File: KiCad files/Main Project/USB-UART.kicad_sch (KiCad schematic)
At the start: 6 parts, among them U3 CH340C

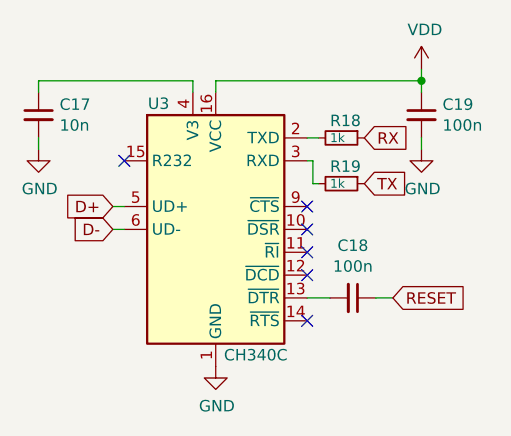
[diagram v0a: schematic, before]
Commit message: shematic update
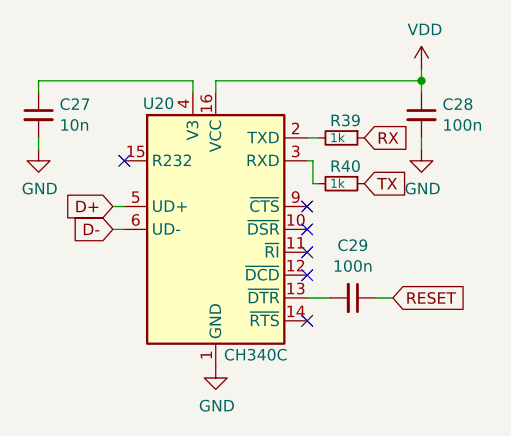
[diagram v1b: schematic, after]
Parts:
- renumbered C17 to C27, C19 to C28, C18 to C29, R18 to R39, R19 to R40, U3 to U20
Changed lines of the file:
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@@
   (symbol (lib_id "Interface_USB:CH340C") (at 140.97 83.82 0) (unit 1)
     (in_bom yes) (on_board yes)
-    (property "Reference" "U3" (id 0) (at 134.62 69.85 0))
+    (property "Reference" "U20" (id 0) (at 134.62 69.85 0))
     (property "Value" "CH340C" (id 1) (at 145.415 97.79 0))
     (property "Footprint" "Package_SO:SOIC-16_3.9x9.9mm_P1.27mm" (id 2) (at 142.24 97.79 0)
@@
   (symbol (lib_id "Device:C_Small") (at 121.285 71.12 0) (unit 1)
     (in_bom yes) (on_board yes)
-    (property "Reference" "C17" (id 0) (at 123.6218 69.9516 0)
+    (property "Reference" "C27" (id 0) (at 123.6218 69.9516 0)
       (effects (font (size 1.27 1.27)) (justify left))
     )
@@
   (symbol (lib_id "power:GND") (at 121.285 74.93 0) (unit 1)
     (in_bom yes) (on_board yes)
-    (property "Reference" "#PWR073" (id 0) (at 121.285 81.28 0)
+    (property "Reference" "#PWR082" (id 0) (at 121.285 81.28 0)
       (effects (font (size 1.27 1.27)) hide)
     )
@@
   (symbol (lib_id "Device:C_Small") (at 163.83 71.12 0) (unit 1)
     (in_bom yes) (on_board yes)
-    (property "Reference" "C19" (id 0) (at 166.1668 69.9516 0)
+    (property "Reference" "C28" (id 0) (at 166.1668 69.9516 0)
       (effects (font (size 1.27 1.27)) (justify left))
     )
@@
   (symbol (lib_id "power:GND") (at 163.83 74.93 0) (unit 1)
     (in_bom yes) (on_board yes)
-    (property "Reference" "#PWR076" (id 0) (at 163.83 81.28 0)
+    (property "Reference" "#PWR083" (id 0) (at 163.83 81.28 0)
       (effects (font (size 1.27 1.27)) hide)
     )
@@
   (symbol (lib_id "power:GND") (at 140.97 99.06 0) (unit 1)
     (in_bom yes) (on_board yes)
-    (property "Reference" "#PWR074" (id 0) (at 140.97 105.41 0)
+    (property "Reference" "#PWR084" (id 0) (at 140.97 105.41 0)
       (effects (font (size 1.27 1.27)) hide)
     )
@@
   (symbol (lib_id "Device:C_Small") (at 156.21 91.44 270) (unit 1)
     (in_bom yes) (on_board yes)
-    (property "Reference" "C18" (id 0) (at 156.21 85.6234 90))
+    (property "Reference" "C29" (id 0) (at 156.21 85.6234 90))
     (property "Value" "100n" (id 1) (at 156.21 87.9348 90))
     (property "Footprint" "Capacitor_SMD:C_0805_2012Metric" (id 2) (at 156.21 91.44 0)
@@
   (symbol (lib_id "Device:R_Small") (at 154.94 73.66 270) (unit 1)
     (in_bom yes) (on_board yes)
-    (property "Reference" "R18" (id 0) (at 153.67 71.755 90)
+    (property "Reference" "R39" (id 0) (at 153.67 71.755 90)
       (effects (font (size 1.27 1.27)) (justify left))
     )
@@
   (symbol (lib_id "Device:R_Small") (at 154.94 78.74 270) (unit 1)
     (in_bom yes) (on_board yes)
-    (property "Reference" "R19" (id 0) (at 153.67 76.835 90)
+    (property "Reference" "R40" (id 0) (at 153.67 76.835 90)
       (effects (font (size 1.27 1.27)) (justify left))
     )
@@
   (symbol (lib_id "power:VDD") (at 163.83 66.04 0) (unit 1)
     (in_bom yes) (on_board yes)
-    (property "Reference" "#PWR075" (id 0) (at 163.83 69.85 0)
+    (property "Reference" "#PWR081" (id 0) (at 163.83 69.85 0)
       (effects (font (size 1.27 1.27)) hide)
     )

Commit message: update
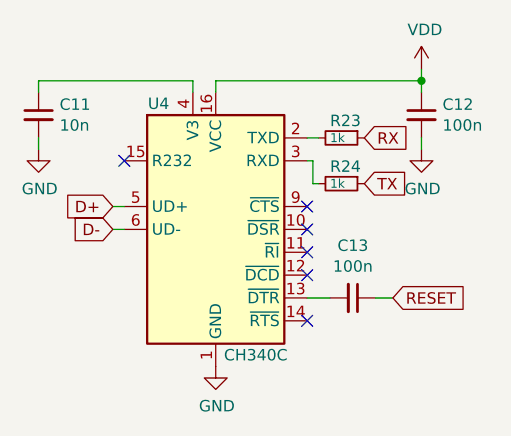
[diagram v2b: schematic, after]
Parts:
- renumbered C27 to C11, C28 to C12, C29 to C13, R39 to R23, R40 to R24, U20 to U4
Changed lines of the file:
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@@
   (symbol (lib_id "Interface_USB:CH340C") (at 140.97 83.82 0) (unit 1)
     (in_bom yes) (on_board yes)
-    (property "Reference" "U20" (id 0) (at 134.62 69.85 0))
+    (property "Reference" "U4" (id 0) (at 134.62 69.85 0))
     (property "Value" "CH340C" (id 1) (at 145.415 97.79 0))
     (property "Footprint" "Package_SO:SOIC-16_3.9x9.9mm_P1.27mm" (id 2) (at 142.24 97.79 0)
@@
   (symbol (lib_id "Device:C_Small") (at 121.285 71.12 0) (unit 1)
     (in_bom yes) (on_board yes)
-    (property "Reference" "C27" (id 0) (at 123.6218 69.9516 0)
+    (property "Reference" "C11" (id 0) (at 123.6218 69.9516 0)
       (effects (font (size 1.27 1.27)) (justify left))
     )
@@
   (symbol (lib_id "power:GND") (at 121.285 74.93 0) (unit 1)
     (in_bom yes) (on_board yes)
-    (property "Reference" "#PWR082" (id 0) (at 121.285 81.28 0)
+    (property "Reference" "#PWR066" (id 0) (at 121.285 81.28 0)
       (effects (font (size 1.27 1.27)) hide)
     )
@@
   (symbol (lib_id "Device:C_Small") (at 163.83 71.12 0) (unit 1)
     (in_bom yes) (on_board yes)
-    (property "Reference" "C28" (id 0) (at 166.1668 69.9516 0)
+    (property "Reference" "C12" (id 0) (at 166.1668 69.9516 0)
       (effects (font (size 1.27 1.27)) (justify left))
     )
@@
   (symbol (lib_id "power:GND") (at 163.83 74.93 0) (unit 1)
     (in_bom yes) (on_board yes)
-    (property "Reference" "#PWR083" (id 0) (at 163.83 81.28 0)
+    (property "Reference" "#PWR067" (id 0) (at 163.83 81.28 0)
       (effects (font (size 1.27 1.27)) hide)
     )
@@
   (symbol (lib_id "power:GND") (at 140.97 99.06 0) (unit 1)
     (in_bom yes) (on_board yes)
-    (property "Reference" "#PWR084" (id 0) (at 140.97 105.41 0)
+    (property "Reference" "#PWR068" (id 0) (at 140.97 105.41 0)
       (effects (font (size 1.27 1.27)) hide)
     )
@@
   (symbol (lib_id "Device:C_Small") (at 156.21 91.44 270) (unit 1)
     (in_bom yes) (on_board yes)
-    (property "Reference" "C29" (id 0) (at 156.21 85.6234 90))
+    (property "Reference" "C13" (id 0) (at 156.21 85.6234 90))
     (property "Value" "100n" (id 1) (at 156.21 87.9348 90))
     (property "Footprint" "Capacitor_SMD:C_0805_2012Metric" (id 2) (at 156.21 91.44 0)
@@
   (symbol (lib_id "Device:R_Small") (at 154.94 73.66 270) (unit 1)
     (in_bom yes) (on_board yes)
-    (property "Reference" "R39" (id 0) (at 153.67 71.755 90)
+    (property "Reference" "R23" (id 0) (at 153.67 71.755 90)
       (effects (font (size 1.27 1.27)) (justify left))
     )
@@
   (symbol (lib_id "Device:R_Small") (at 154.94 78.74 270) (unit 1)
     (in_bom yes) (on_board yes)
-    (property "Reference" "R40" (id 0) (at 153.67 76.835 90)
+    (property "Reference" "R24" (id 0) (at 153.67 76.835 90)
       (effects (font (size 1.27 1.27)) (justify left))
     )
@@
   (symbol (lib_id "power:VDD") (at 163.83 66.04 0) (unit 1)
     (in_bom yes) (on_board yes)
-    (property "Reference" "#PWR081" (id 0) (at 163.83 69.85 0)
+    (property "Reference" "#PWR065" (id 0) (at 163.83 69.85 0)
       (effects (font (size 1.27 1.27)) hide)
     )

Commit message: update
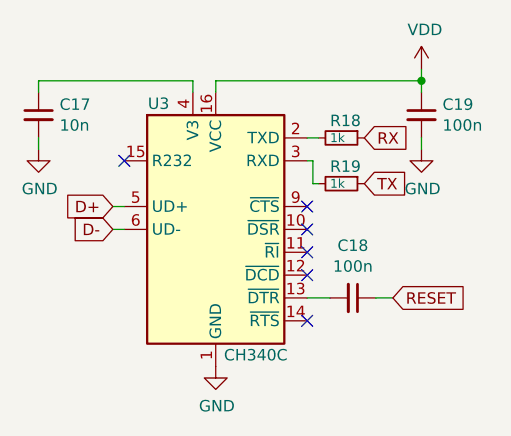
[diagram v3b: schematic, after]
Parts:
- renumbered C11 to C17, C13 to C18, C12 to C19, R23 to R18, R24 to R19, U4 to U3
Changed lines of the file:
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@@
   (symbol (lib_id "Interface_USB:CH340C") (at 140.97 83.82 0) (unit 1)
     (in_bom yes) (on_board yes)
-    (property "Reference" "U4" (id 0) (at 134.62 69.85 0))
+    (property "Reference" "U3" (id 0) (at 134.62 69.85 0))
     (property "Value" "CH340C" (id 1) (at 145.415 97.79 0))
     (property "Footprint" "Package_SO:SOIC-16_3.9x9.9mm_P1.27mm" (id 2) (at 142.24 97.79 0)
@@
   (symbol (lib_id "Device:C_Small") (at 121.285 71.12 0) (unit 1)
     (in_bom yes) (on_board yes)
-    (property "Reference" "C11" (id 0) (at 123.6218 69.9516 0)
+    (property "Reference" "C17" (id 0) (at 123.6218 69.9516 0)
       (effects (font (size 1.27 1.27)) (justify left))
     )
@@
   (symbol (lib_id "power:GND") (at 121.285 74.93 0) (unit 1)
     (in_bom yes) (on_board yes)
-    (property "Reference" "#PWR066" (id 0) (at 121.285 81.28 0)
+    (property "Reference" "#PWR073" (id 0) (at 121.285 81.28 0)
       (effects (font (size 1.27 1.27)) hide)
     )
@@
   (symbol (lib_id "Device:C_Small") (at 163.83 71.12 0) (unit 1)
     (in_bom yes) (on_board yes)
-    (property "Reference" "C12" (id 0) (at 166.1668 69.9516 0)
+    (property "Reference" "C19" (id 0) (at 166.1668 69.9516 0)
       (effects (font (size 1.27 1.27)) (justify left))
     )
@@
   (symbol (lib_id "power:GND") (at 163.83 74.93 0) (unit 1)
     (in_bom yes) (on_board yes)
-    (property "Reference" "#PWR067" (id 0) (at 163.83 81.28 0)
+    (property "Reference" "#PWR076" (id 0) (at 163.83 81.28 0)
       (effects (font (size 1.27 1.27)) hide)
     )
@@
   (symbol (lib_id "power:GND") (at 140.97 99.06 0) (unit 1)
     (in_bom yes) (on_board yes)
-    (property "Reference" "#PWR068" (id 0) (at 140.97 105.41 0)
+    (property "Reference" "#PWR074" (id 0) (at 140.97 105.41 0)
       (effects (font (size 1.27 1.27)) hide)
     )
@@
   (symbol (lib_id "Device:C_Small") (at 156.21 91.44 270) (unit 1)
     (in_bom yes) (on_board yes)
-    (property "Reference" "C13" (id 0) (at 156.21 85.6234 90))
+    (property "Reference" "C18" (id 0) (at 156.21 85.6234 90))
     (property "Value" "100n" (id 1) (at 156.21 87.9348 90))
     (property "Footprint" "Capacitor_SMD:C_0805_2012Metric" (id 2) (at 156.21 91.44 0)
@@
   (symbol (lib_id "Device:R_Small") (at 154.94 73.66 270) (unit 1)
     (in_bom yes) (on_board yes)
-    (property "Reference" "R23" (id 0) (at 153.67 71.755 90)
+    (property "Reference" "R18" (id 0) (at 153.67 71.755 90)
       (effects (font (size 1.27 1.27)) (justify left))
     )
@@
   (symbol (lib_id "Device:R_Small") (at 154.94 78.74 270) (unit 1)
     (in_bom yes) (on_board yes)
-    (property "Reference" "R24" (id 0) (at 153.67 76.835 90)
+    (property "Reference" "R19" (id 0) (at 153.67 76.835 90)
       (effects (font (size 1.27 1.27)) (justify left))
     )
@@
   (symbol (lib_id "power:VDD") (at 163.83 66.04 0) (unit 1)
     (in_bom yes) (on_board yes)
-    (property "Reference" "#PWR065" (id 0) (at 163.83 69.85 0)
+    (property "Reference" "#PWR075" (id 0) (at 163.83 69.85 0)
       (effects (font (size 1.27 1.27)) hide)
     )
